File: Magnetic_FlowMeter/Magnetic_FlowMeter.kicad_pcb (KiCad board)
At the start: 2 copper layers, 101.6 x 53.3 mm, 13 parts, among them P1 Digital, P10 CONN_01X01, P11 CONN_01X01, P12 CONN_01X01, P13 CONN_01X01, P2 Power, P3 Analog, P4 Analog, P5 PWM, P6 PWM, P7 Communication, P8 CONN_01X01, P9 CONN_01X01

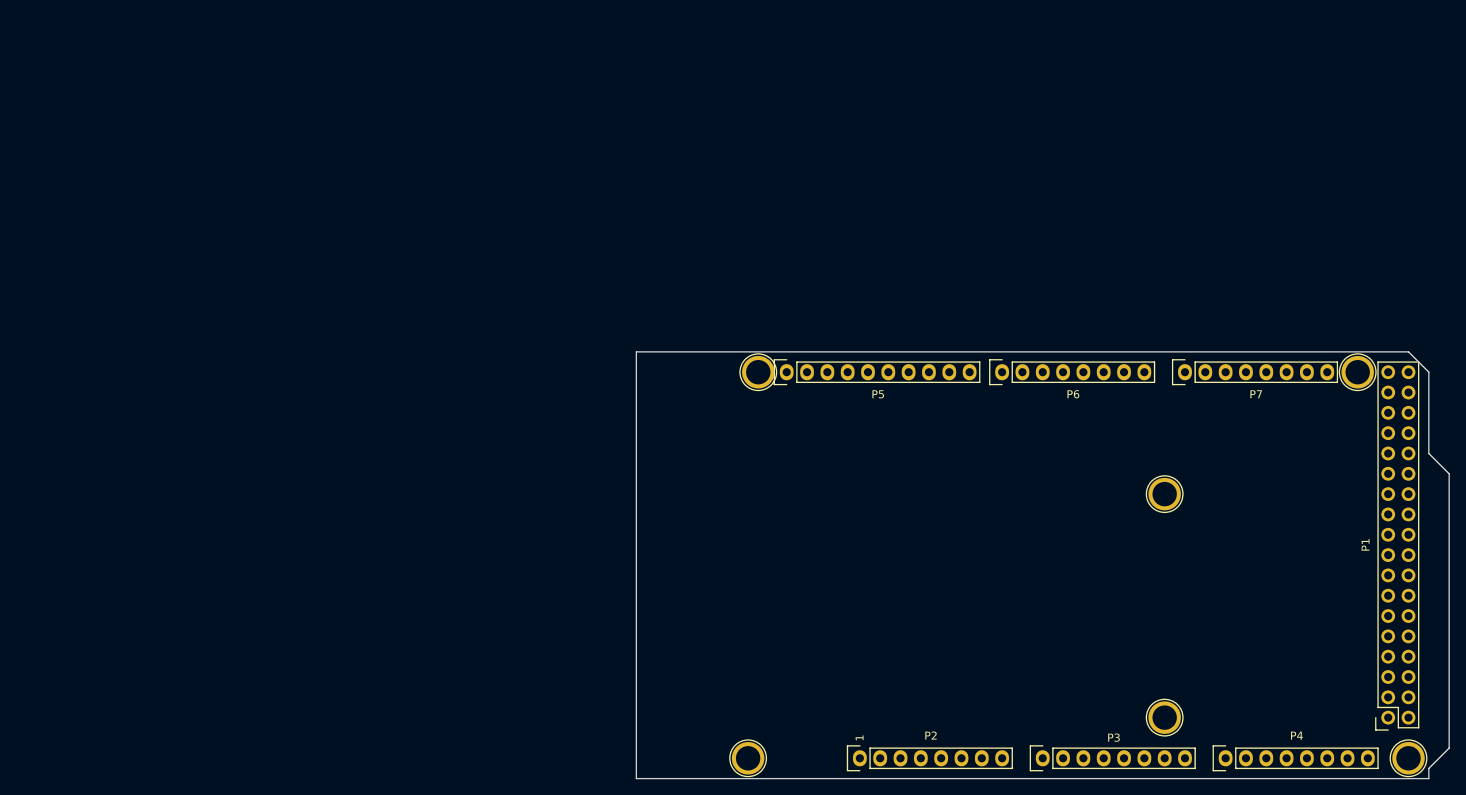
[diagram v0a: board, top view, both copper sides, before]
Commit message: Update
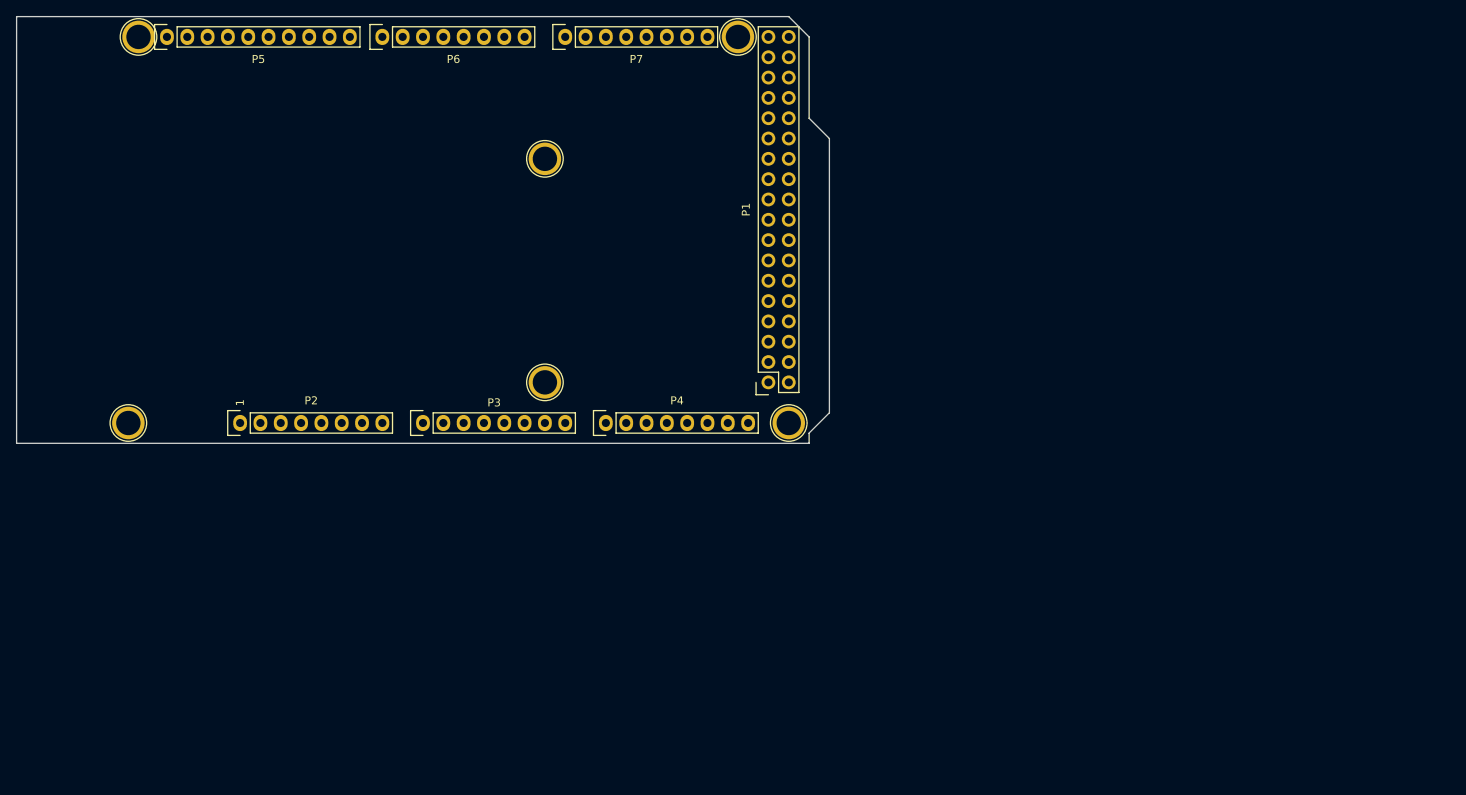
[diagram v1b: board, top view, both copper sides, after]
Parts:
- moved P8 88.1 mm to (117.3, 119.1)
- moved P10 88.1 mm to (199.9, 119.1)
- moved P11 88.1 mm to (118.6, 70.9)
- moved P12 88.1 mm to (169.4, 86.1)
- moved P2 88.1 mm to (131.3, 119.1)
- moved P3 88.1 mm to (154.2, 119.1)
- moved P4 88.1 mm to (177.0, 119.1)
- moved P5 88.1 mm to (122.2, 70.9)
- moved P6 88.1 mm to (149.1, 70.9)
- moved P7 88.1 mm to (172.0, 70.9)
- moved P9 88.1 mm to (169.4, 114.0)
- moved P13 88.1 mm to (193.5, 70.9)
- moved P1 88.1 mm to (197.4, 114.0)
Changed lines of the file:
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@@
-(kicad_pcb (version 4) (host pcbnew 4.0.7-e1-6374~58~ubuntu16.04.1)
+(kicad_pcb (version 4) (host pcbnew 4.0.2-4+6225~38~ubuntu14.04.1-stable)
   (general
     (links 6)
     (no_connects 6)
-    (area 96.952999 66.843 205.053001 122.995)
+    (area 103.302999 68.250999 205.053001 121.741001)
     (thickness 1.6)
     (drawings 27)
@@
   )
   (module Socket_Arduino_Mega:Socket_Strip_Arduino_2x18 locked (layer F.Cu)
-    (at 274.828 155.956 90)
+    (at 197.358 114.046 90)
     (descr "Through hole socket strip")
     (tags "socket strip")
@@
   )
   (module Socket_Arduino_Mega:Socket_Strip_Arduino_1x08 locked (layer F.Cu)
-    (at 208.788 161.036)
+    (at 131.318 119.126)
     (descr "Through hole socket strip")
     (tags "socket strip")
@@
   )
   (module Socket_Arduino_Mega:Socket_Strip_Arduino_1x08 locked (layer F.Cu)
-    (at 231.648 161.036)
+    (at 154.178 119.126)
     (descr "Through hole socket strip")
     (tags "socket strip")
@@
   )
   (module Socket_Arduino_Mega:Socket_Strip_Arduino_1x08 locked (layer F.Cu)
-    (at 254.508 161.036)
+    (at 177.038 119.126)
     (descr "Through hole socket strip")
     (tags "socket strip")
@@
   )
   (module Socket_Arduino_Mega:Socket_Strip_Arduino_1x10 locked (layer F.Cu)
-    (at 199.644 112.776)
+    (at 122.174 70.866)
     (descr "Through hole socket strip")
     (tags "socket strip")
@@
   )
   (module Socket_Arduino_Mega:Socket_Strip_Arduino_1x08 locked (layer F.Cu)
-    (at 226.568 112.776)
+    (at 149.098 70.866)
     (descr "Through hole socket strip")
     (tags "socket strip")
@@
   )
   (module Socket_Arduino_Mega:Socket_Strip_Arduino_1x08 locked (layer F.Cu)
-    (at 249.428 112.776)
+    (at 171.958 70.866)
     (descr "Through hole socket strip")
     (tags "socket strip")
@@
   )
   (module Socket_Arduino_Mega:Arduino_1pin locked (layer F.Cu)
-    (at 194.818 161.036)
+    (at 117.348 119.126)
     (descr "module 1 pin (ou trou mecanique de percage)")
     (tags DEV)
@@
   )
   (module Socket_Arduino_Mega:Arduino_1pin locked (layer F.Cu)
-    (at 246.888 155.956)
+    (at 169.418 114.046)
     (descr "module 1 pin (ou trou mecanique de percage)")
     (tags DEV)
@@
   )
   (module Socket_Arduino_Mega:Arduino_1pin locked (layer F.Cu)
-    (at 277.368 161.036)
+    (at 199.898 119.126)
     (descr "module 1 pin (ou trou mecanique de percage)")
     (tags DEV)
@@
   )
   (module Socket_Arduino_Mega:Arduino_1pin locked (layer F.Cu)
-    (at 196.088 112.776)
+    (at 118.618 70.866)
     (descr "module 1 pin (ou trou mecanique de percage)")
     (tags DEV)
@@
   )
   (module Socket_Arduino_Mega:Arduino_1pin locked (layer F.Cu)
-    (at 246.888 128.016)
+    (at 169.418 86.106)
     (descr "module 1 pin (ou trou mecanique de percage)")
     (tags DEV)
@@
   )
   (module Socket_Arduino_Mega:Arduino_1pin locked (layer F.Cu)
-    (at 271.018 112.776)
+    (at 193.548 70.866)
     (descr "module 1 pin (ou trou mecanique de percage)")
     (tags DEV)
@@
       (net 76 "Net-(P13-Pad1)"))
   )
-  (gr_text 1 (at 208.788 158.496 90) (layer F.SilkS)
+  (gr_text 1 (at 131.318 116.586 90) (layer F.SilkS)
     (effects (font (size 1 1) (thickness 0.15)))
   )
-  (gr_line (start 253.0856 138.684) (end 253.0856 132.6388) (angle 90) (layer Dwgs.User) (width 0.15))
-  (gr_line (start 256.9464 138.684) (end 256.9464 132.6388) (angle 90) (layer Dwgs.User) (width 0.15))
-  (gr_line (start 253.0856 138.684) (end 256.9464 138.684) (angle 90) (layer Dwgs.User) (width 0.15))
-  (gr_circle (center 255.016 135.636) (end 256.286 135.636) (layer Dwgs.User) (width 0.15))
-  (gr_line (start 253.0856 132.6388) (end 256.9464 132.6388) (angle 90) (layer Dwgs.User) (width 0.15))
-  (gr_line (start 243.205 139.446) (end 243.205 131.826) (angle 90) (layer Dwgs.User) (width 0.15))
-  (gr_line (start 248.285 139.446) (end 243.205 139.446) (angle 90) (layer Dwgs.User) (width 0.15))
-  (gr_line (start 248.285 131.826) (end 248.285 139.446) (angle 90) (layer Dwgs.User) (width 0.15))
-  (gr_line (start 243.205 131.826) (end 248.285 131.826) (angle 90) (layer Dwgs.User) (width 0.15))
-  (gr_line (start 174.498 131.191) (end 174.498 119.761) (angle 90) (layer Dwgs.User) (width 0.15))
-  (gr_line (start 190.373 131.191) (end 174.498 131.191) (angle 90) (layer Dwgs.User) (width 0.15))
-  (gr_line (start 190.373 119.761) (end 190.373 131.191) (angle 90) (layer Dwgs.User) (width 0.15))
-  (gr_line (start 174.498 119.761) (end 190.373 119.761) (angle 90) (layer Dwgs.User) (width 0.15))
-  (gr_line (start 178.943 160.401) (end 178.943 151.511) (angle 90) (layer Dwgs.User) (width 0.15))
-  (gr_line (start 192.278 160.401) (end 178.943 160.401) (angle 90) (layer Dwgs.User) (width 0.15))
-  (gr_line (start 192.278 151.511) (end 192.278 160.401) (angle 90) (layer Dwgs.User) (width 0.15))
-  (gr_line (start 178.943 151.511) (end 192.278 151.511) (angle 90) (layer Dwgs.User) (width 0.15))
-  (gr_line (start 279.908 163.576) (end 180.848 163.576) (angle 90) (layer Edge.Cuts) (width 0.15))
-  (gr_line (start 279.908 162.306) (end 279.908 163.576) (angle 90) (layer Edge.Cuts) (width 0.15))
-  (gr_line (start 282.448 159.766) (end 279.908 162.306) (angle 90) (layer Edge.Cuts) (width 0.15))
-  (gr_line (start 282.448 125.476) (end 282.448 159.766) (angle 90) (layer Edge.Cuts) (width 0.15))
-  (gr_line (start 279.908 122.936) (end 282.448 125.476) (angle 90) (layer Edge.Cuts) (width 0.15))
-  (gr_line (start 279.908 112.776) (end 279.908 122.936) (angle 90) (layer Edge.Cuts) (width 0.15))
-  (gr_line (start 277.368 110.236) (end 279.908 112.776) (angle 90) (layer Edge.Cuts) (width 0.15))
-  (gr_line (start 180.848 110.236) (end 277.368 110.236) (angle 90) (layer Edge.Cuts) (width 0.15))
-  (gr_line (start 180.848 163.576) (end 180.848 110.236) (angle 90) (layer Edge.Cuts) (width 0.15))
+  (gr_line (start 175.6156 96.774) (end 175.6156 90.7288) (angle 90) (layer Dwgs.User) (width 0.15))
+  (gr_line (start 179.4764 96.774) (end 179.4764 90.7288) (angle 90) (layer Dwgs.User) (width 0.15))
+  (gr_line (start 175.6156 96.774) (end 179.4764 96.774) (angle 90) (layer Dwgs.User) (width 0.15))
+  (gr_circle (center 177.546 93.726) (end 178.816 93.726) (layer Dwgs.User) (width 0.15))
+  (gr_line (start 175.6156 90.7288) (end 179.4764 90.7288) (angle 90) (layer Dwgs.User) (width 0.15))
+  (gr_line (start 165.735 97.536) (end 165.735 89.916) (angle 90) (layer Dwgs.User) (width 0.15))
+  (gr_line (start 170.815 97.536) (end 165.735 97.536) (angle 90) (layer Dwgs.User) (width 0.15))
+  (gr_line (start 170.815 89.916) (end 170.815 97.536) (angle 90) (layer Dwgs.User) (width 0.15))
+  (gr_line (start 165.735 89.916) (end 170.815 89.916) (angle 90) (layer Dwgs.User) (width 0.15))
+  (gr_line (start 97.028 89.281) (end 97.028 77.851) (angle 90) (layer Dwgs.User) (width 0.15))
+  (gr_line (start 112.903 89.281) (end 97.028 89.281) (angle 90) (layer Dwgs.User) (width 0.15))
+  (gr_line (start 112.903 77.851) (end 112.903 89.281) (angle 90) (layer Dwgs.User) (width 0.15))
+  (gr_line (start 97.028 77.851) (end 112.903 77.851) (angle 90) (layer Dwgs.User) (width 0.15))
+  (gr_line (start 101.473 118.491) (end 101.473 109.601) (angle 90) (layer Dwgs.User) (width 0.15))
+  (gr_line (start 114.808 118.491) (end 101.473 118.491) (angle 90) (layer Dwgs.User) (width 0.15))
+  (gr_line (start 114.808 109.601) (end 114.808 118.491) (angle 90) (layer Dwgs.User) (width 0.15))
+  (gr_line (start 101.473 109.601) (end 114.808 109.601) (angle 90) (layer Dwgs.User) (width 0.15))
+  (gr_line (start 202.438 121.666) (end 103.378 121.666) (angle 90) (layer Edge.Cuts) (width 0.15))
+  (gr_line (start 202.438 120.396) (end 202.438 121.666) (angle 90) (layer Edge.Cuts) (width 0.15))
+  (gr_line (start 204.978 117.856) (end 202.438 120.396) (angle 90) (layer Edge.Cuts) (width 0.15))
+  (gr_line (start 204.978 83.566) (end 204.978 117.856) (angle 90) (layer Edge.Cuts) (width 0.15))
+  (gr_line (start 202.438 81.026) (end 204.978 83.566) (angle 90) (layer Edge.Cuts) (width 0.15))
+  (gr_line (start 202.438 70.866) (end 202.438 81.026) (angle 90) (layer Edge.Cuts) (width 0.15))
+  (gr_line (start 199.898 68.326) (end 202.438 70.866) (angle 90) (layer Edge.Cuts) (width 0.15))
+  (gr_line (start 103.378 68.326) (end 199.898 68.326) (angle 90) (layer Edge.Cuts) (width 0.15))
+  (gr_line (start 103.378 121.666) (end 103.378 68.326) (angle 90) (layer Edge.Cuts) (width 0.15))
 )
